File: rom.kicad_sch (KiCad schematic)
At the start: 3 parts, among them IC18 74ACT08, U8 28C256

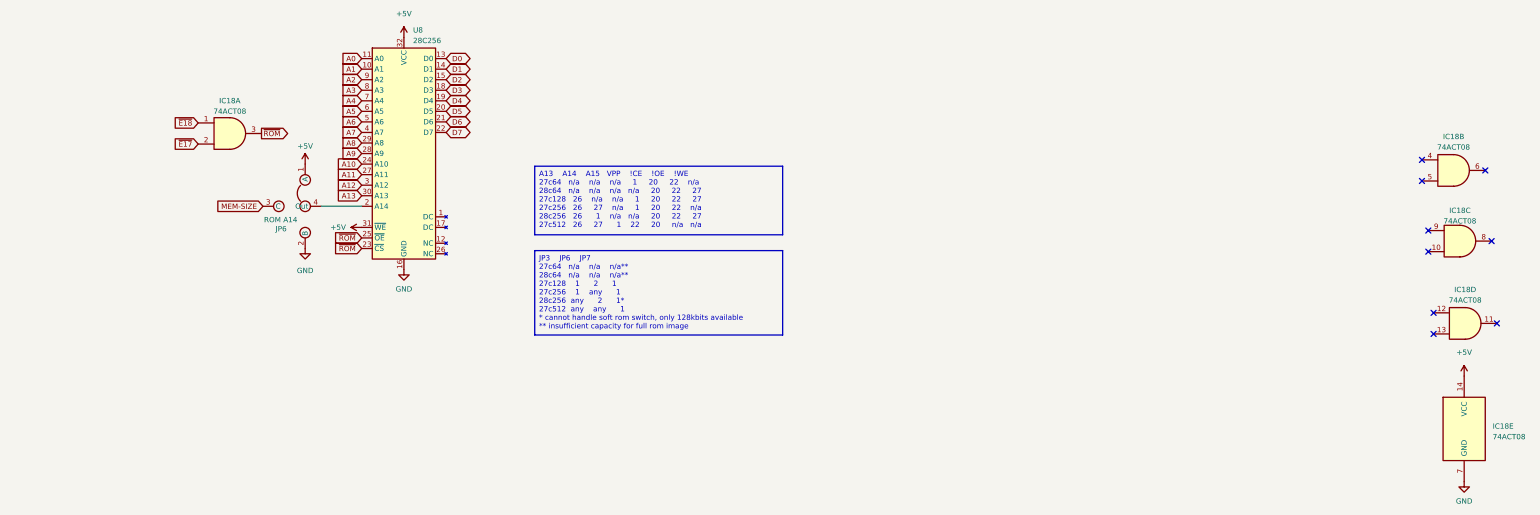
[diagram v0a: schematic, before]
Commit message: serial wiring
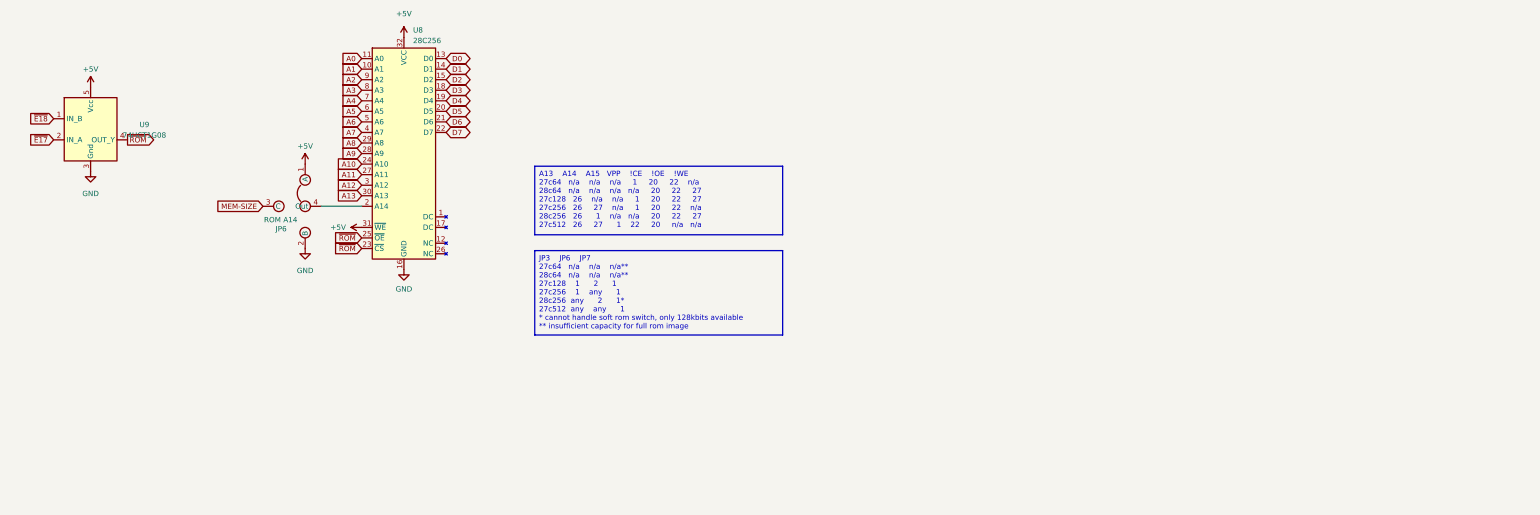
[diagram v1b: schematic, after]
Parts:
- removed IC18: 74ACT08, Package_SO:SOIC-14_3.9x8.7mm_P1.27mm, symbol 74xx:74LS08
- added U9: 74HCT1G08, Package_TO_SOT_SMD:SOT-353_SC-70-5_Handsoldering, symbol vdg:74HC1G08
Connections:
- net +5V: now also U9.5 (Vcc)
- net GND: now also U9.3 (Gnd)
- net ~{E17}: now also U9.2 (IN_A)
- net ~{E18}: now also U9.1 (IN_B)
- net ~{ROM}: now also U9.4 (OUT_Y)
- no-connect marks 9 -> 0
